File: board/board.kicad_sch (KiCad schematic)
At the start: 1 part

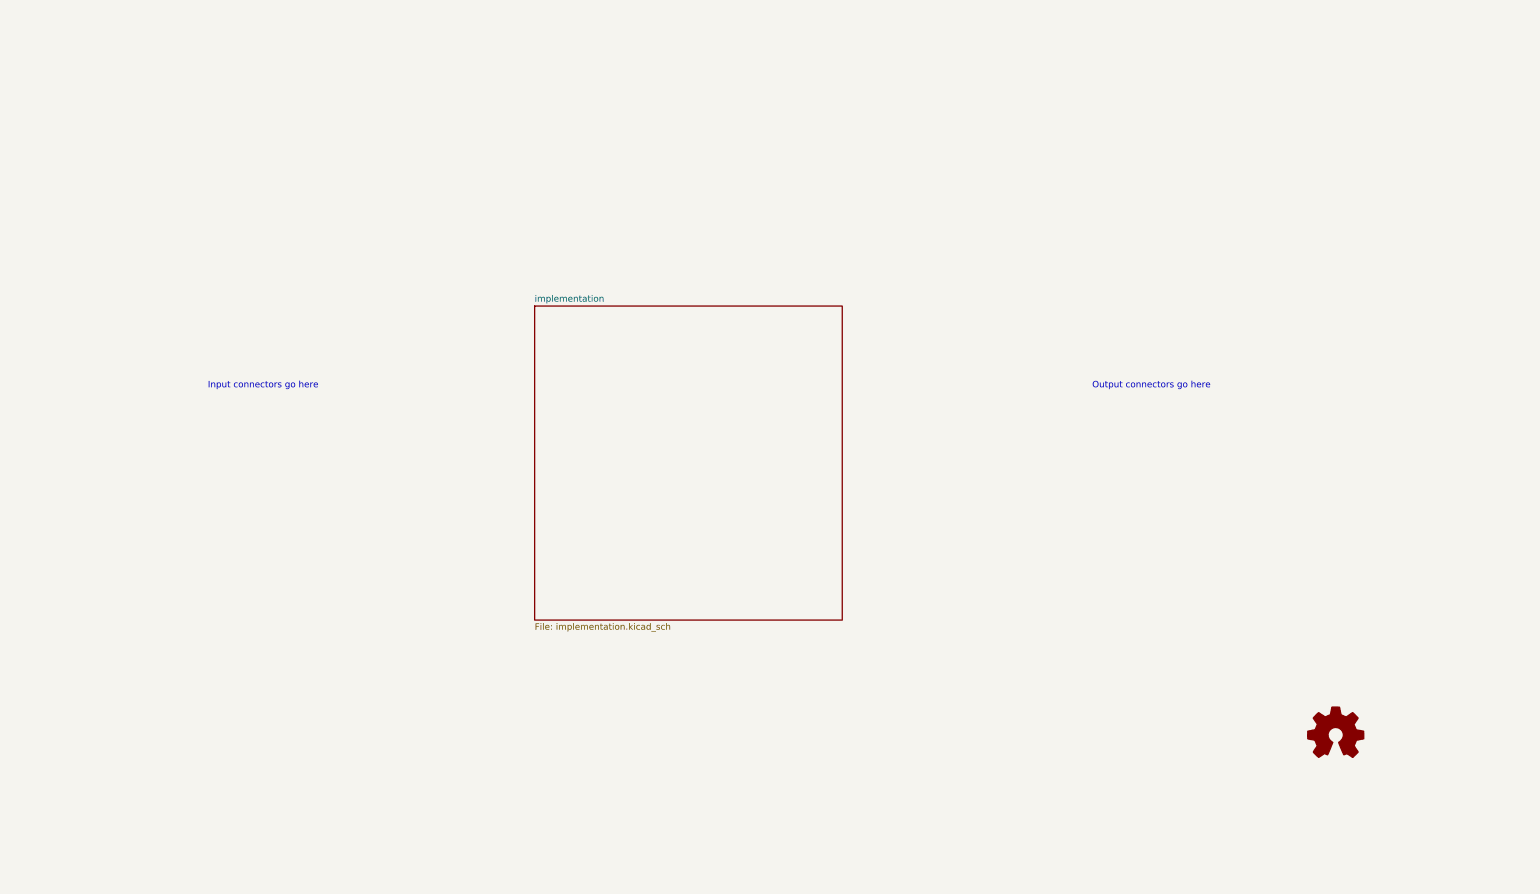
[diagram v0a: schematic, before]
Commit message: updated schemetic and layout
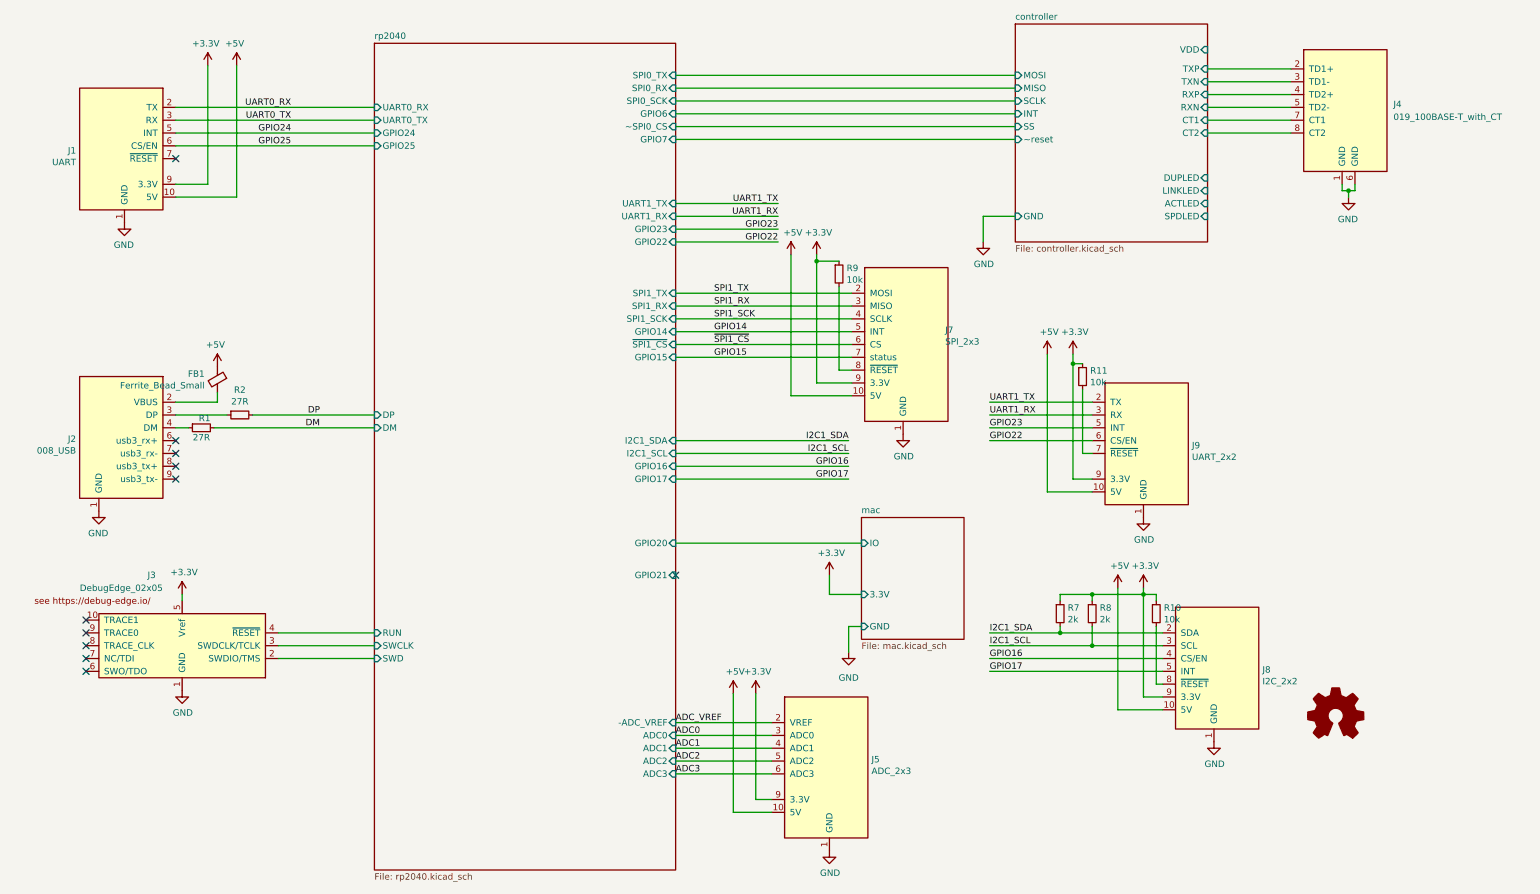
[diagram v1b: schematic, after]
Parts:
- added FB1: Ferrite_Bead_Small, Inductor_SMD:L_0805_2012Metric, symbol Device:FerriteBead_Small
- added J1: UART, on_edge:on_edge_2x05_device, symbol put_on_edge:010_UART
- added J2: 008_USB, on_edge:on_edge_2x05_device, symbol put_on_edge:008_USB
- added J3: DebugEdge_02x05, on_edge:debug_edge_2x05_device, symbol put_on_edge:DebugEdge_02x05
- added J4: 019_100BASE-T_with_CT, on_edge:on_edge_2x05_host, symbol put_on_edge:019_100BASE-T_with_CT
- added J5: ADC_2x3, on_edge:on_edge_2x05_host, symbol put_on_edge:007_ADC
- added J7: SPI_2x3, on_edge:on_edge_2x05_host, symbol put_on_edge:002_SPI
- added J8: I2C_2x2, on_edge:on_edge_2x05_host, symbol put_on_edge:001_I2C
- added J9: UART_2x2, on_edge:on_edge_2x05_host, symbol put_on_edge:010_UART
- added R1, R2: 27R, Resistor_SMD:R_0603_1608Metric, symbol Device:R_Small
- added R10, R11, R9: 10k, Resistor_SMD:R_0603_1608Metric, symbol Device:R_Small
- added R7, R8: 2k, Resistor_SMD:R_0603_1608Metric, symbol Device:R_Small
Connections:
- new net: J9.7 (~{RESET}), R11.2
- new net: J7.8 (~{RESET}), R9.2
- new net: J2.4 (DM), R1.1
- new net: J8.8 (~{RESET}), R10.2
- new net: J2.3 (DP), R2.1
- new net: FB1.2, J2.2 (VBUS)
- new net +3V3: J1.9 (3.3V), J3.5 (Vref), J5.9 (3.3V), J7.9 (3.3V), J8.9 (3.3V), J9.9 (3.3V), R10.1, R11.1, R7.1, R8.1, R9.1
- new net +5V: FB1.1, J1.10 (5V), J5.10 (5V), J7.10 (5V), J8.10 (5V), J9.10 (5V)
- new net ADC0: J5.3 (ADC0)
- new net ADC1: J5.4 (ADC1)
- new net ADC2: J5.5 (ADC2)
- new net ADC3: J5.6 (ADC3)
- new net ADC_VREF: J5.2 (VREF)
- new net DM: R1.2
- new net DP: R2.2
- new net GND: J1.1 (GND), J2.1 (GND), J3.1 (GND), J4.1 (GND), J4.6 (GND), J5.1 (GND), J7.1 (GND), J8.1 (GND), J9.1 (GND)
- new net GPIO14: J7.5 (INT)
- new net GPIO15: J7.7 (status)
- new net GPIO16: J8.4 (CS/EN)
- new net GPIO17: J8.5 (INT)
- new net GPIO22: J9.6 (CS/EN)
- new net GPIO23: J9.5 (INT)
- new net GPIO24: J1.5 (INT)
- new net GPIO25: J1.6 (CS/EN)
- new net I2C1_SCL: J8.3 (SCL), R8.2
- new net I2C1_SDA: J8.2 (SDA), R7.2
- new net SPI1_RX: J7.3 (MISO)
- new net SPI1_SCK: J7.4 (SCLK)
- new net SPI1_TX: J7.2 (MOSI)
- new net UART0_RX: J1.2 (TX)
- new net UART0_TX: J1.3 (RX)
- new net UART1_RX: J9.3 (RX)
- new net UART1_TX: J9.2 (TX)
- new net controller/CT1: J4.7 (CT1)
- new net controller/CT2: J4.8 (CT2)
- new net controller/RXN: J4.5 (TD2-)
- new net controller/RXP: J4.4 (TD2+)
- new net controller/TXN: J4.3 (TD1-)
- new net controller/TXP: J4.2 (TD1+)
- new net rp2040/RUN: J3.4 (~{RESET})
- new net rp2040/SWCLK: J3.3 (SWDCLK/TCLK)
- new net rp2040/SWD: J3.2 (SWDIO/TMS)
- new net ~{SPI1_CS}: J7.6 (CS)
- no-connect marks 0 -> 11
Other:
- sheet implementation renamed rp2040
- added sheet controller (controller.kicad_sch)
- added sheet mac (mac.kicad_sch)
- sheet rp2040: file implementation.kicad_sch -> rp2040.kicad_sch
- sheet rp2040 ports: added ADC0, ADC1, ADC2, ADC3, DM, DP, GPIO14, GPIO15, GPIO16, GPIO17, GPIO20, GPIO21, GPIO22, GPIO23, GPIO24, GPIO25, GPIO6, GPIO7, I2C1_SCL, I2C1_SDA, RUN, SPI0_RX, SPI0_SCK, SPI0_TX, SPI1_RX, SPI1_SCK, SPI1_TX, SWCLK, SWD, UART0_RX, UART0_TX, UART1_RX, UART1_TX, ~SPI0_CS, ~{SPI1_CS}, ­ADC_VREF; removed none
- note removed: "Input connectors go here"
- note removed: "Output connectors go here"
